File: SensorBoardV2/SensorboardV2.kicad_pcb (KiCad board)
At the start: 2 copper layers, 158.3 x 29.7 mm, 63 parts, among them J1 Conn_01x16_Pin, U1 LM339, U10 LM339, U2 CNY70, U3 CNY70, U4 CNY70, U5 CNY70, U6 CNY70, U7 CNY70, U8 CNY70

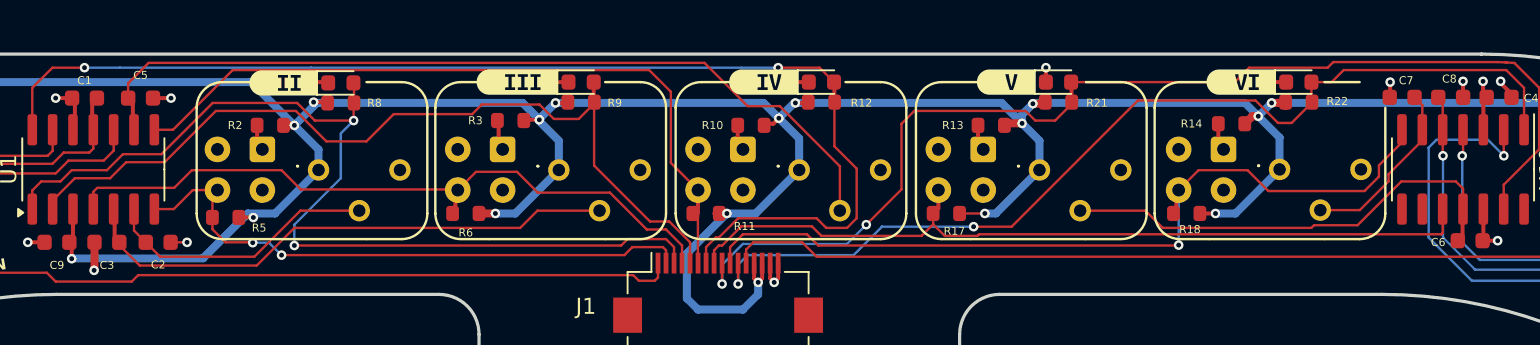
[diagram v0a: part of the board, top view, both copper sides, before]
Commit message: Final Update
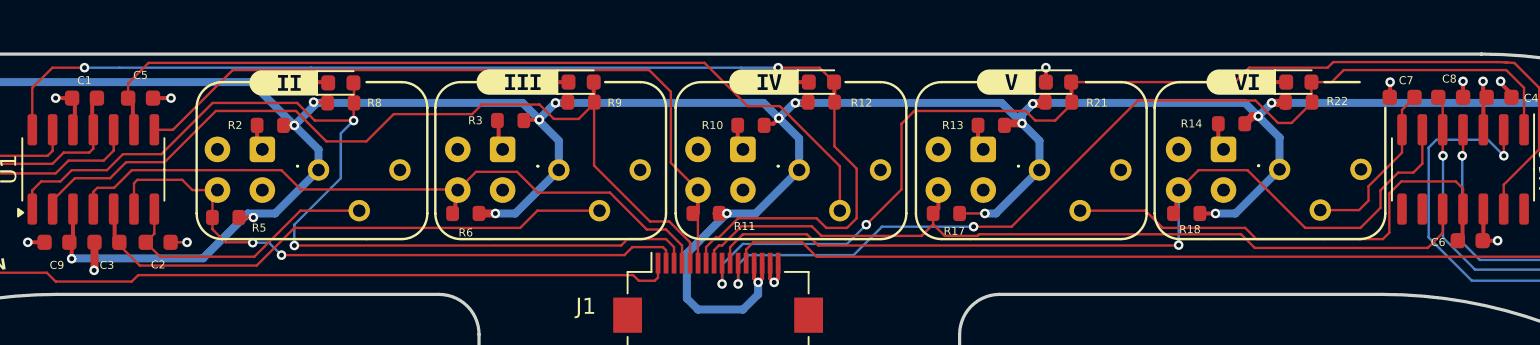
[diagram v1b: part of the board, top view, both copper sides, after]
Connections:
- C2 pad 1: Net-(U1B--) -> Net-(U1B-+)
- C7 pad 1: Net-(U10B--) -> Net-(U10B-+)
- RV2 pad 2: Net-(U1B--) -> Net-(U1B-+)
- RV6 pad 2: Net-(U10B--) -> Net-(U10B-+)
- U1 pad 6: Net-(U1B--) -> /IR_2_A
- U1 pad 7: /IR_2_A -> Net-(U1B-+)
- U10 pad 6: Net-(U10B--) -> /IR_6_A
- U10 pad 7: /IR_6_A -> Net-(U10B-+)
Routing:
- net Net-(U1B--): track 17.3 -> 0.00 mm
- net Net-(U1B-+): track 0.00 -> 17.2 mm
- net Net-(U10B--): track 11.3 -> 0.00 mm
- net Net-(U10B-+): track 0.00 -> 10.9 mm
- net /IR_6_A: track 52.1 -> 56.3 mm
- net /IR_2_A: track 37.1 -> 39.9 mm
- net Net-(U10C-+): track 28.8 -> 30.8 mm
- net /IR_5_A: track 51.7 -> 52.4 mm
